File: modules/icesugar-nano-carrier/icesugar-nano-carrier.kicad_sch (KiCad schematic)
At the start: 3 parts, among them J1 Conn_01x06_Pin, J2 Conn_01x06_Pin, J3 Conn_02x06_Odd_Even

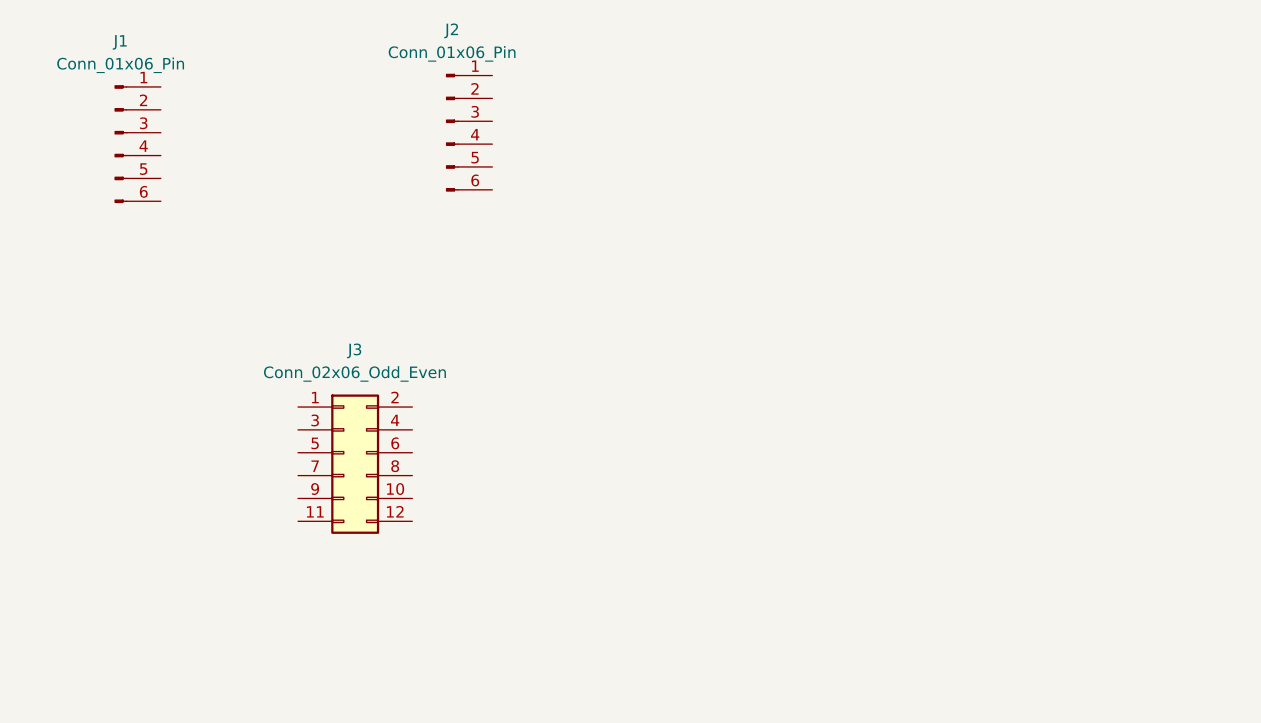
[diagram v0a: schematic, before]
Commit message: finish ICESugar Nano carrier board design
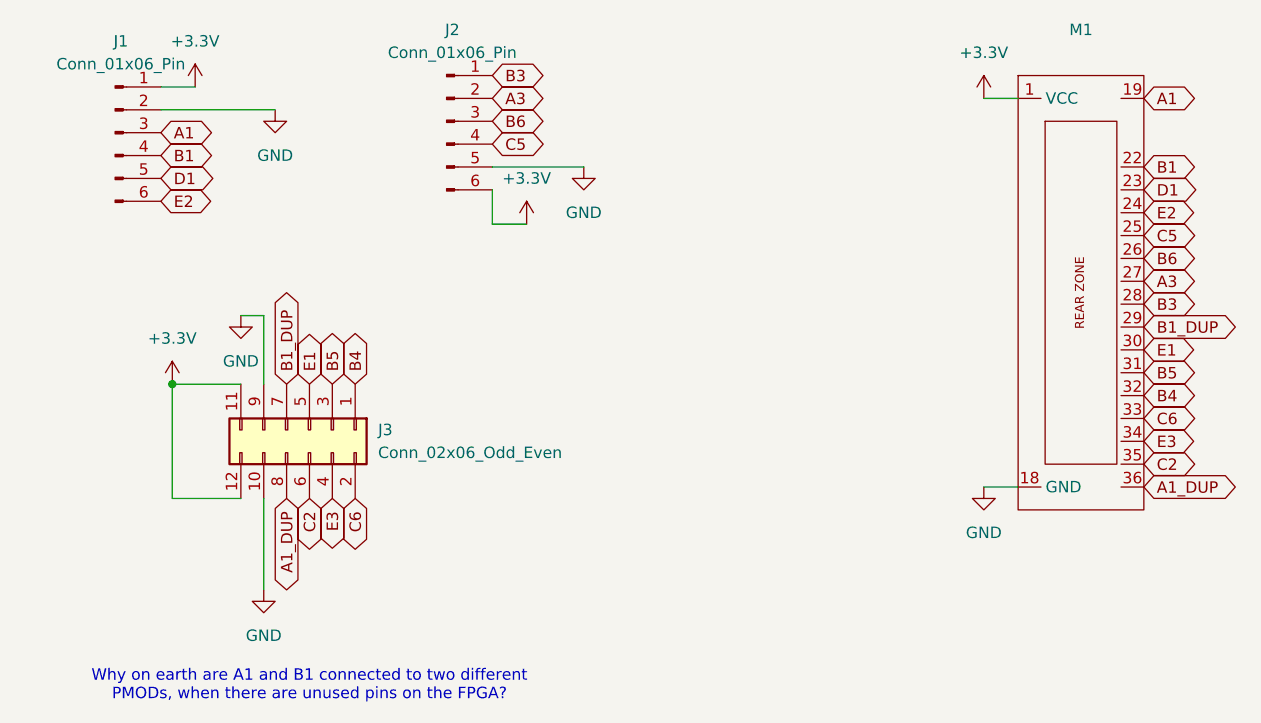
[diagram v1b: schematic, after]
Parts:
- added M1: ~, MegaCastle:MegaCastle2x18-Module-I24.0x40.9-M800067FFF, symbol MegaCastle:MegaCastle2x18-Module-I24.0x40.9-M800067FFF
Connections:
- net +3.3V: now reaches J1.1 (Pin_1)
- net +3.3V: now also J2.6 (Pin_6), J3.11 (Pin_11), J3.12 (Pin_12), M1.1 (VCC)
- net GND: now reaches J1.2 (Pin_2)
- net GND: now also J2.5 (Pin_5), J3.10 (Pin_10), J3.9 (Pin_9), M1.18 (GND)
- net A1: now reaches J1.3 (Pin_3)
- net A1: now also M1.19
- net B1: now reaches J1.4 (Pin_4)
- net B1: now also M1.22
- net D1: now reaches J1.5 (Pin_5)
- net D1: now also M1.23
- net E2: now reaches J1.6 (Pin_6)
- net E2: now also M1.24
- net B4: now reaches J3.1 (Pin_1)
- net B4: now also M1.32
- net C6: now reaches J3.2 (Pin_2)
- net C6: now also M1.33
- net B5: now reaches J3.3 (Pin_3)
- net B5: now also M1.31
- net E3: now reaches J3.4 (Pin_4)
- net E3: now also M1.34
- net E1: now reaches J3.5 (Pin_5)
- net E1: now also M1.30
- net C2: now reaches J3.6 (Pin_6)
- net C2: now also M1.35
- net B1_DUP: now reaches J3.7 (Pin_7)
- net B1_DUP: now also M1.29
- net A1_DUP: now reaches J3.8 (Pin_8)
- net A1_DUP: now also M1.36
- net B3: now reaches J2.1 (Pin_1)
- net B3: now also M1.28
- net A3: now reaches J2.2 (Pin_2)
- net A3: now also M1.27
- net B6: now reaches J2.3 (Pin_3)
- net B6: now also M1.26
- net C5: now reaches J2.4 (Pin_4)
- net C5: now also M1.25
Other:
- note added: "Why on earth are A1 and B1 connected to two different PMODs, when there are unused pins on the FPGA?"
- moved on the sheet: J3
